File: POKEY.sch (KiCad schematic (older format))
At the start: 59 parts, among them J201 Diagnostic, U22 POKEY, U24 CD4051B, U25 CD4051B

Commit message: Almost finished
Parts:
- R74: footprint Atari:R_Axial_DIN0207_L3.6mm_D2.2mm_P10.16mm_Horizontal -> Resistor_SMD:R_1206_3216Metric_Pad1.42x1.75mm_HandSolder
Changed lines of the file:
@@
 F 0 "R74" V 7375 1475 50  0000 C CNN
 F 1 "3k" V 7425 1625 50  0000 C CNN
-F 2 "Atari:R_Axial_DIN0207_L3.6mm_D2.2mm_P10.16mm_Horizontal" V 7305 1475 50  0001 C CNN
+F 2 "Resistor_SMD:R_1206_3216Metric_Pad1.42x1.75mm_HandSolder" V 7305 1475 50  0001 C CNN
 F 3 "~" H 7375 1475 50  0001 C CNN
 	1    7375 1475

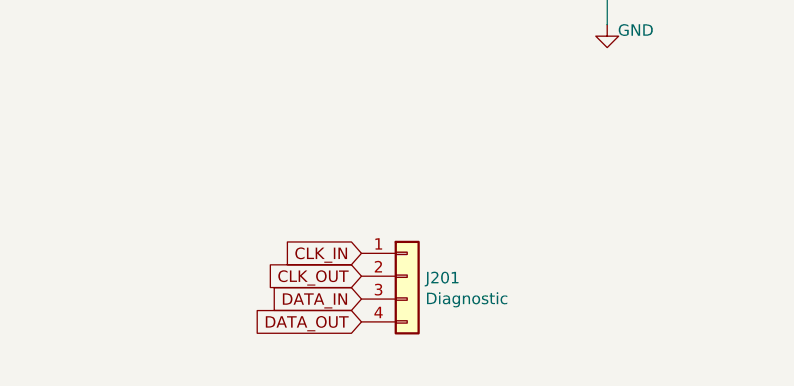
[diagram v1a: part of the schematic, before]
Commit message: SIO2SD schema
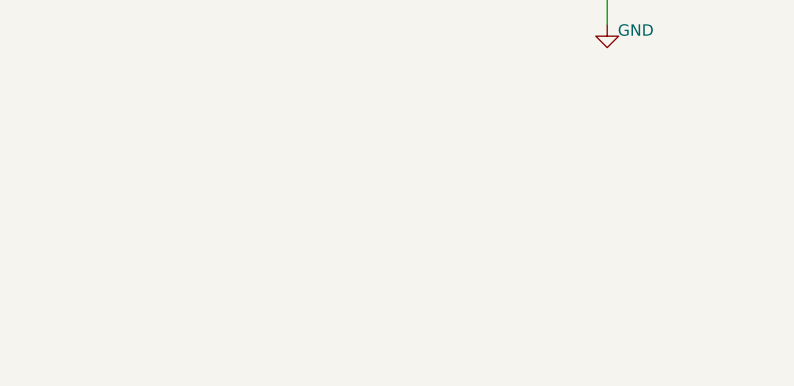
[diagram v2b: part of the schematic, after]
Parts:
- removed J201: Diagnostic, Connector_PinHeader_2.54mm:PinHeader_1x04_P2.54mm_Vertical, symbol Connector_Generic:Conn_01x04
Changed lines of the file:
@@
 $Descr A4 11693 8268
 encoding utf-8
-Sheet 11 16
+Sheet 11 17
 Title ""
 Date ""
@@
 Wire Wire Line
 	5400 5700 5675 5700
-$Comp
-L Connector_Generic:Conn_01x04 J201
-U 1 1 604341BE
-P 2425 6050
-F 0 "J201" H 2505 6042 50  0000 L CNN
-F 1 "Diagnostic" H 2505 5951 50  0000 L CNN
-F 2 "Connector_PinHeader_2.54mm:PinHeader_1x04_P2.54mm_Vertical" H 2425 6050 50  0001 C CNN
-F 3 "~" H 2425 6050 50  0001 C CNN
-	1    2425 6050
-	1    0    0    -1
-$EndComp
-Text GLabel 2225 6050 0    50   Input ~ 0
-CLK_OUT
-Text GLabel 2225 5950 0    50   Input ~ 0
-CLK_IN
-Text GLabel 2225 6150 0    50   Input ~ 0
-DATA_IN
-Text GLabel 2225 6250 0    50   Input ~ 0
-DATA_OUT
 Wire Wire Line
 	3300 3600 3300 3700
